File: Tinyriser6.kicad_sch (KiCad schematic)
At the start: 25 parts, among them J1 Bus_M.2_Socket_M, J2 Bus_PCI_Express_x16, J3 Conn_02x04_Odd_Even, M1 Fan_4pin

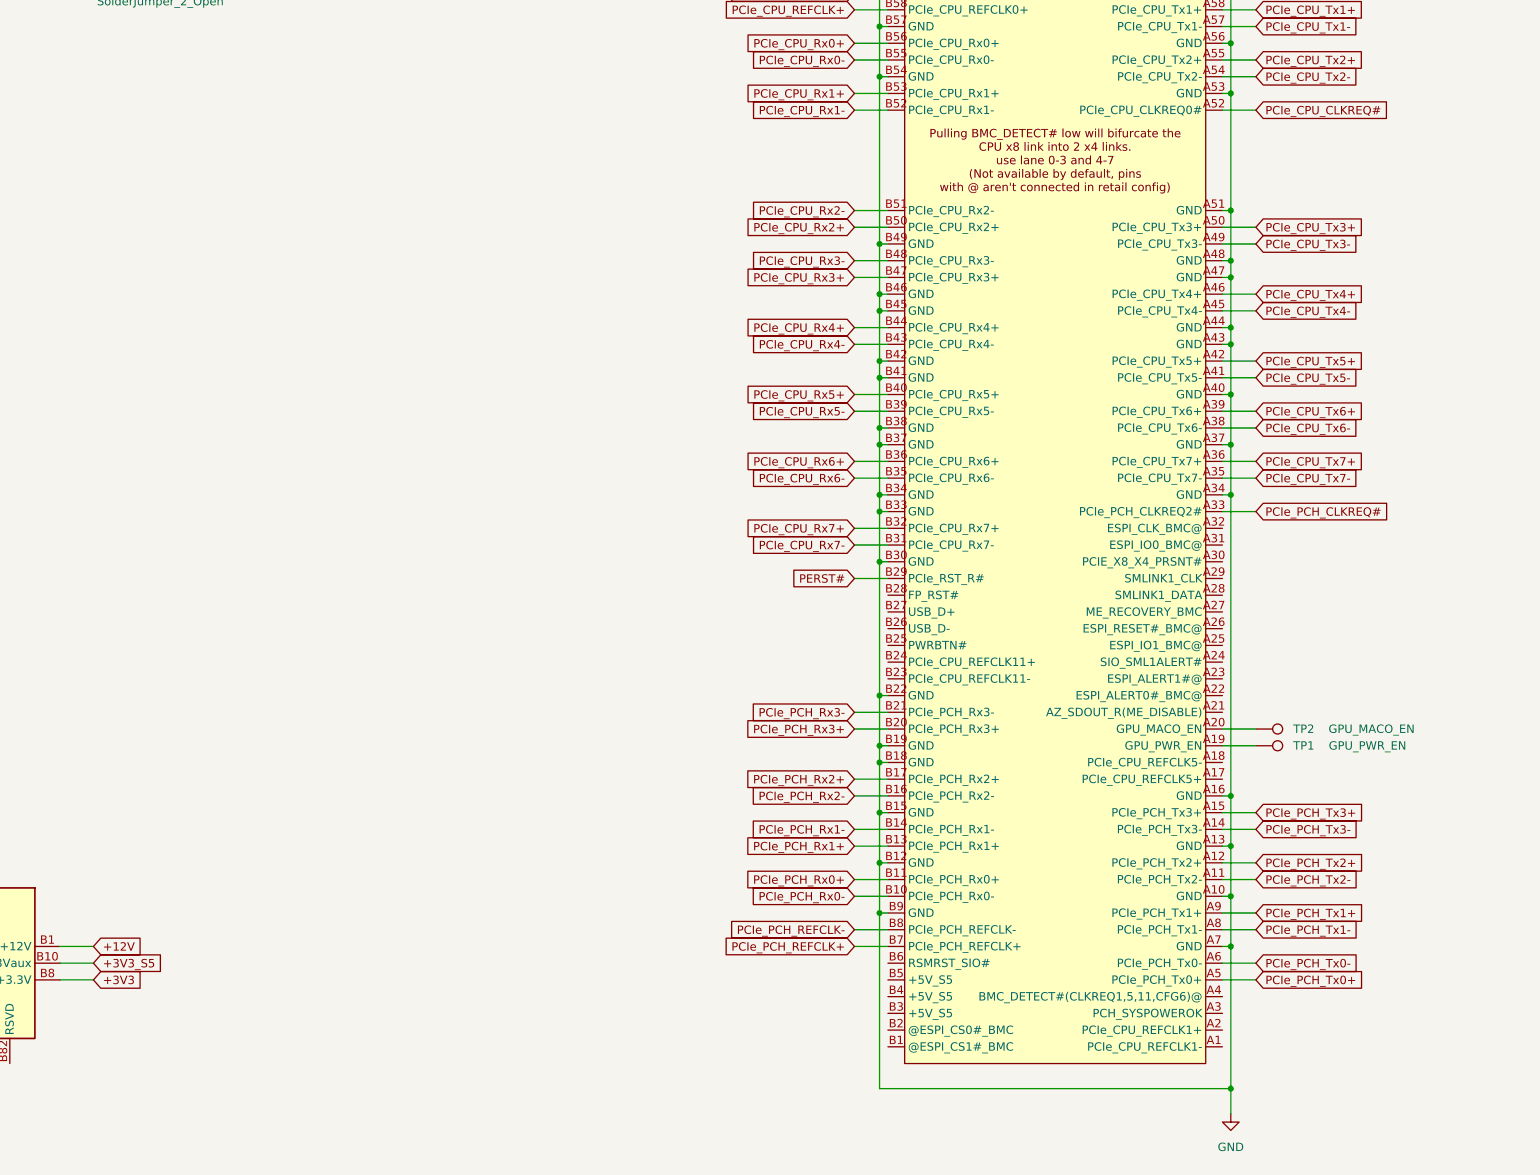
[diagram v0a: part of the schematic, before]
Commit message: started breaking out all the weird pins
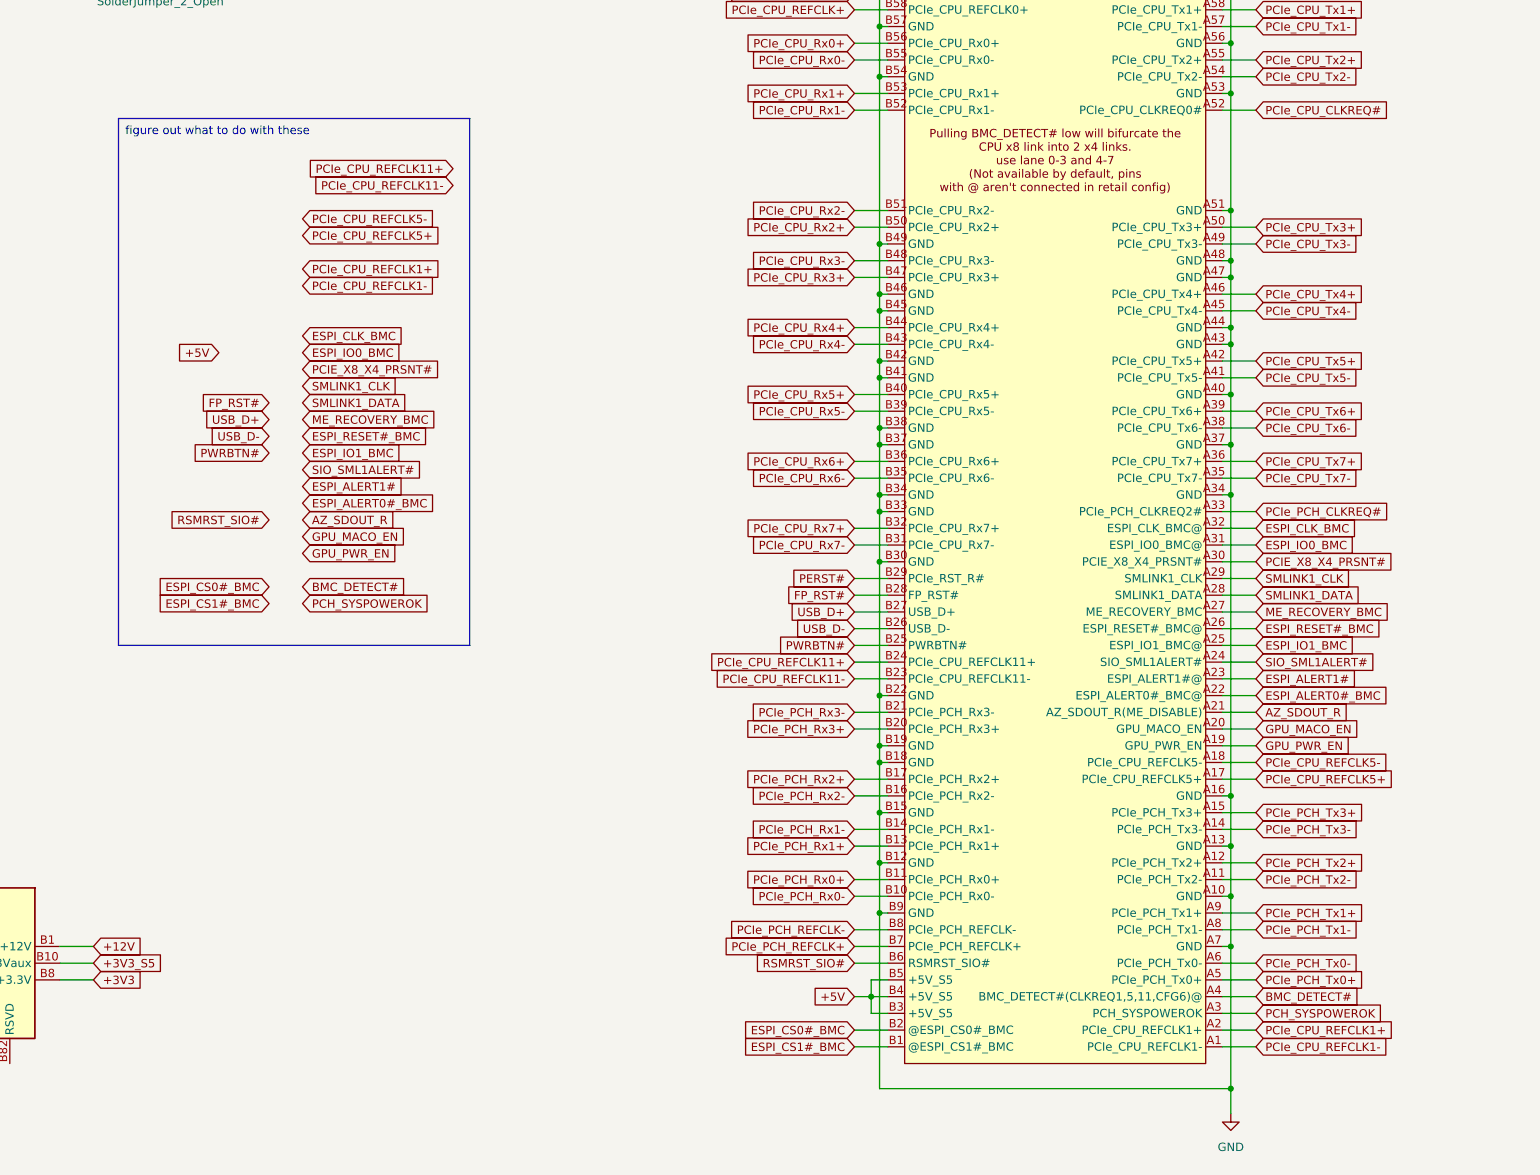
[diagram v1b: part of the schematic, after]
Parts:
- removed TP1: GPU_PWR_EN, TestPoint:TestPoint_Pad_D1.0mm, symbol Connector:TestPoint
- removed TP2: GPU_MACO_EN, TestPoint:TestPoint_Pad_D1.0mm, symbol Connector:TestPoint
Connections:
- net PCIe_CPU_REFCLK1-: now reaches J4.A1 (PCIe_CPU_REFCLK1-)
- net PCIe_CPU_REFCLK5+: now reaches J4.A17 (PCIe_CPU_REFCLK5+)
- net PCIe_CPU_REFCLK5-: now reaches J4.A18 (PCIe_CPU_REFCLK5-)
- net GPU_PWR_EN: now reaches J4.A19 (GPU_PWR_EN)
- net PCIe_CPU_REFCLK1+: now reaches J4.A2 (PCIe_CPU_REFCLK1+)
- net GPU_MACO_EN: now reaches J4.A20 (GPU_MACO_EN)
- net AZ_SDOUT_R: now reaches J4.A21 (AZ_SDOUT_R(ME_DISABLE))
- net ESPI_ALERT0#_BMC: now reaches J4.A22 (ESPI_ALERT0#_BMC@)
- net ESPI_ALERT1#: now reaches J4.A23 (ESPI_ALERT1#@)
- net SIO_SML1ALERT#: now reaches J4.A24 (SIO_SML1ALERT#)
- net ESPI_IO1_BMC: now reaches J4.A25 (ESPI_IO1_BMC@)
- net ESPI_RESET#_BMC: now reaches J4.A26 (ESPI_RESET#_BMC@)
- net ME_RECOVERY_BMC: now reaches J4.A27 (ME_RECOVERY_BMC)
- net SMLINK1_DATA: now reaches J4.A28 (SMLINK1_DATA)
- net SMLINK1_CLK: now reaches J4.A29 (SMLINK1_CLK)
- net PCH_SYSPOWEROK: now reaches J4.A3 (PCH_SYSPOWEROK)
- net PCIE_X8_X4_PRSNT#: now reaches J4.A30 (PCIE_X8_X4_PRSNT#)
- net ESPI_IO0_BMC: now reaches J4.A31 (ESPI_IO0_BMC@)
- net ESPI_CLK_BMC: now reaches J4.A32 (ESPI_CLK_BMC@)
- net BMC_DETECT#: now reaches J4.A4 (BMC_DETECT#(CLKREQ1,5,11,CFG6)@)
- net ESPI_CS1#_BMC: now reaches J4.B1 (@ESPI_CS1#_BMC)
- net ESPI_CS0#_BMC: now reaches J4.B2 (@ESPI_CS0#_BMC)
- net PCIe_CPU_REFCLK11-: now reaches J4.B23 (PCIe_CPU_REFCLK11-)
- net PCIe_CPU_REFCLK11+: now reaches J4.B24 (PCIe_CPU_REFCLK11+)
- net PWRBTN#: now reaches J4.B25 (PWRBTN#)
- net USB_D-: now reaches J4.B26 (USB_D-)
- net USB_D+: now reaches J4.B27 (USB_D+)
- net FP_RST#: now reaches J4.B28 (FP_RST#)
- net +5V: now reaches J4.B3 (+5V_S5)
- net +5V: now also J4.B4 (+5V_S5), J4.B5 (+5V_S5)
- net RSMRST_SIO#: now reaches J4.B6 (RSMRST_SIO#)
